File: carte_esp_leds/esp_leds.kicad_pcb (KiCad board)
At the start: 2 copper layers, 27 x 47 mm, 16 parts, among them J1 LEDs, J2 Prog, J3 USB_B_Mini, SW1 SW_Push, U1 BPC_ESP8266-01_ESP-01, U2 AMS1117-3.3, U3 74AHCT1G125

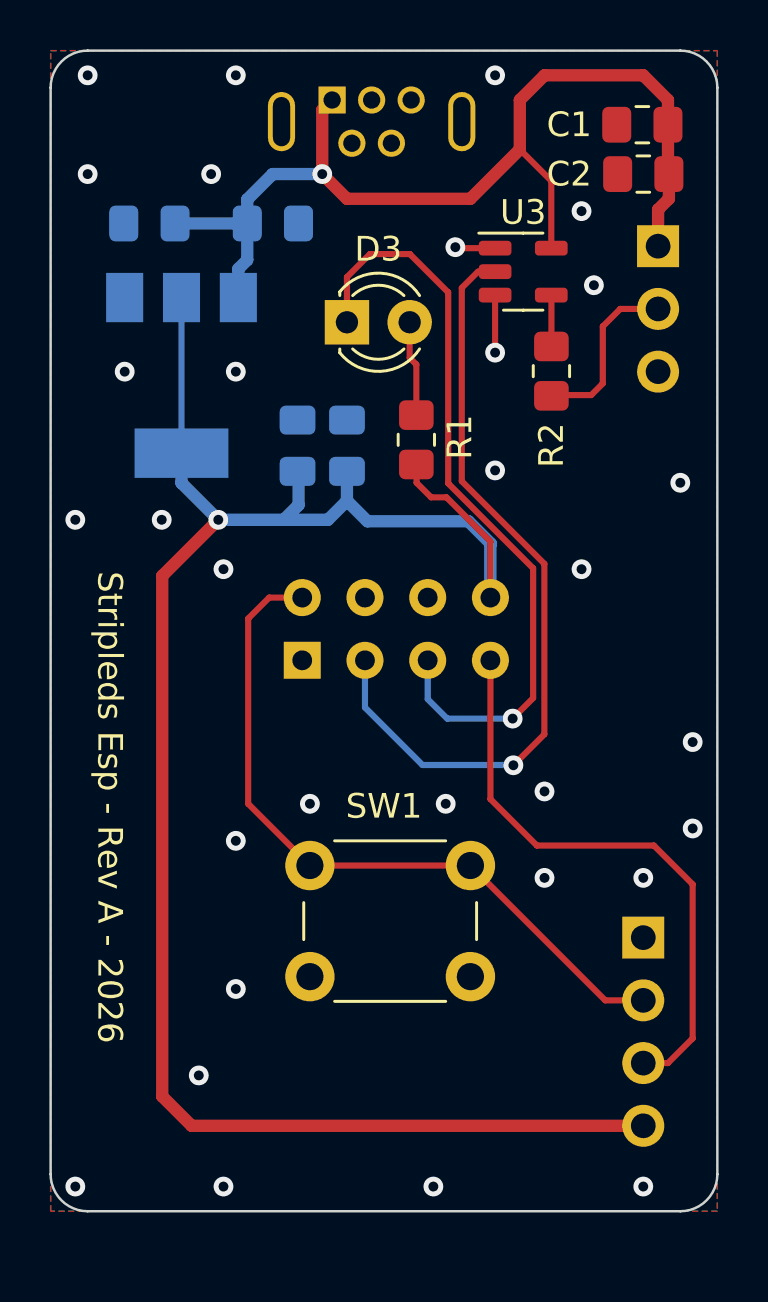
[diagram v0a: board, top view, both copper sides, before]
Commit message: Finalisation
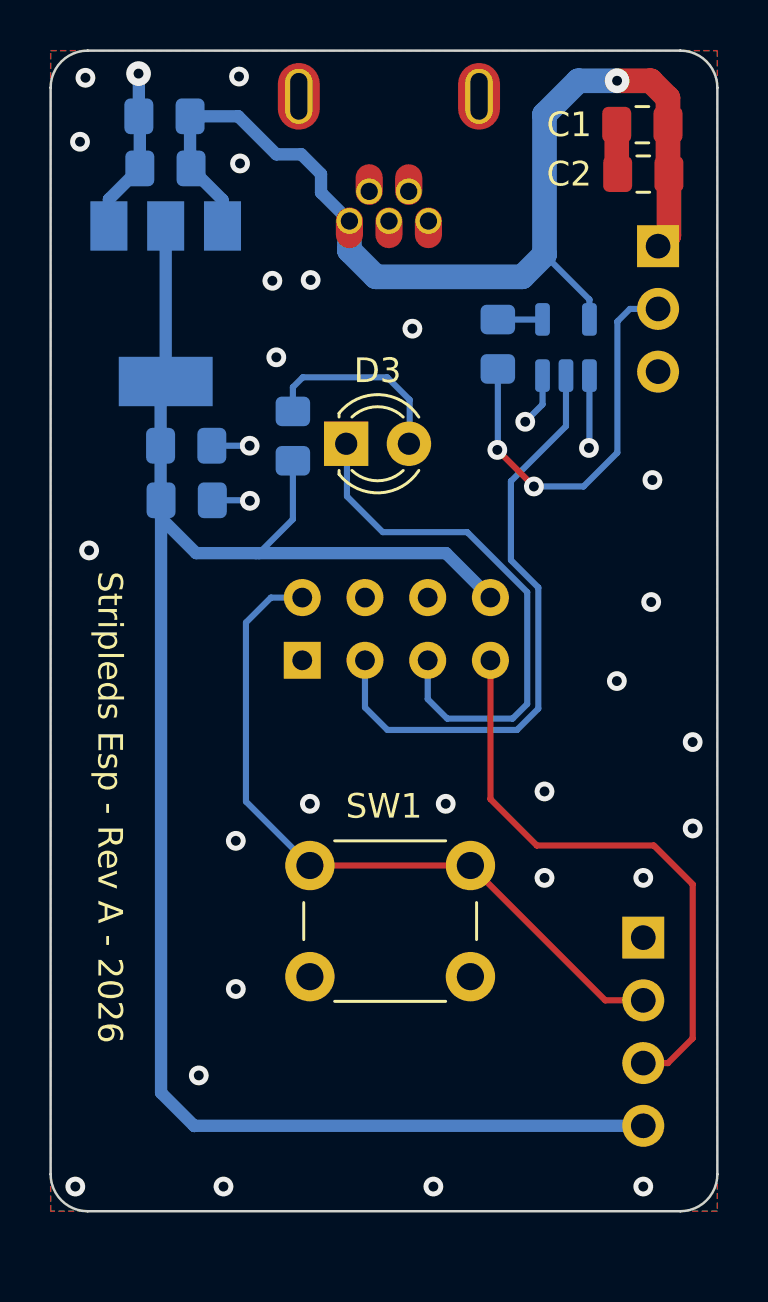
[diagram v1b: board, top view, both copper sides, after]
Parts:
- J3: value USB_B_Mini -> 54819-0519; footprint Connector_USB:USB_Mini-B_Tensility_54-00023_Vertical -> bpc:BPC_MiniUsb_Molex_54819-0519
- R1, R2, U3: moved to B.Cu
- moved C5 6.86 mm to (135.5, 72.2), turned to 180 degrees
- moved C3 6.17 mm to (134.6, 56.7), turned to 0 degrees
- moved R1 5.00 mm to (139.8, 69.6)
- moved J3 4.95 mm to (142.1, 60.9)
- moved D3 4.92 mm to (142.0, 69.9)
- moved C6 4.51 mm to (135.5, 70.0), turned to 0 degrees
- moved U3 3.53 mm to (150.9, 66.0), turned to 90 degrees
- moved U2 2.97 mm to (134.7, 64.2)
- moved R2 2.43 mm to (148.1, 65.9)
- moved C4 2.32 mm to (134.7, 58.8)
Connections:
- J3 pad 6: GND -> +5V
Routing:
- net GND: track 3.96 -> 16.9 mm
- net Net-(D3-K): track 31.3 -> 21.7 mm, vias 1 -> 0
- net Net-(J1-Pin_2): track 7.13 -> 16.5 mm, vias 0 -> 2
- net DATA: track 31.7 -> 24.5 mm, vias 1 -> 0
- net Net-(D3-A): track 3.87 -> 8.11 mm
- net +3.3V: track 78.6 -> 75.0 mm, vias 1 -> 0
- net +5V: track 42.4 -> 44.6 mm
